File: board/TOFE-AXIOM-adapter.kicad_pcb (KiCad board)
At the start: 4 copper layers, 68.9 x 28.3 mm, 11 parts, among them CN1 C, U1 24AA01/24LC01B

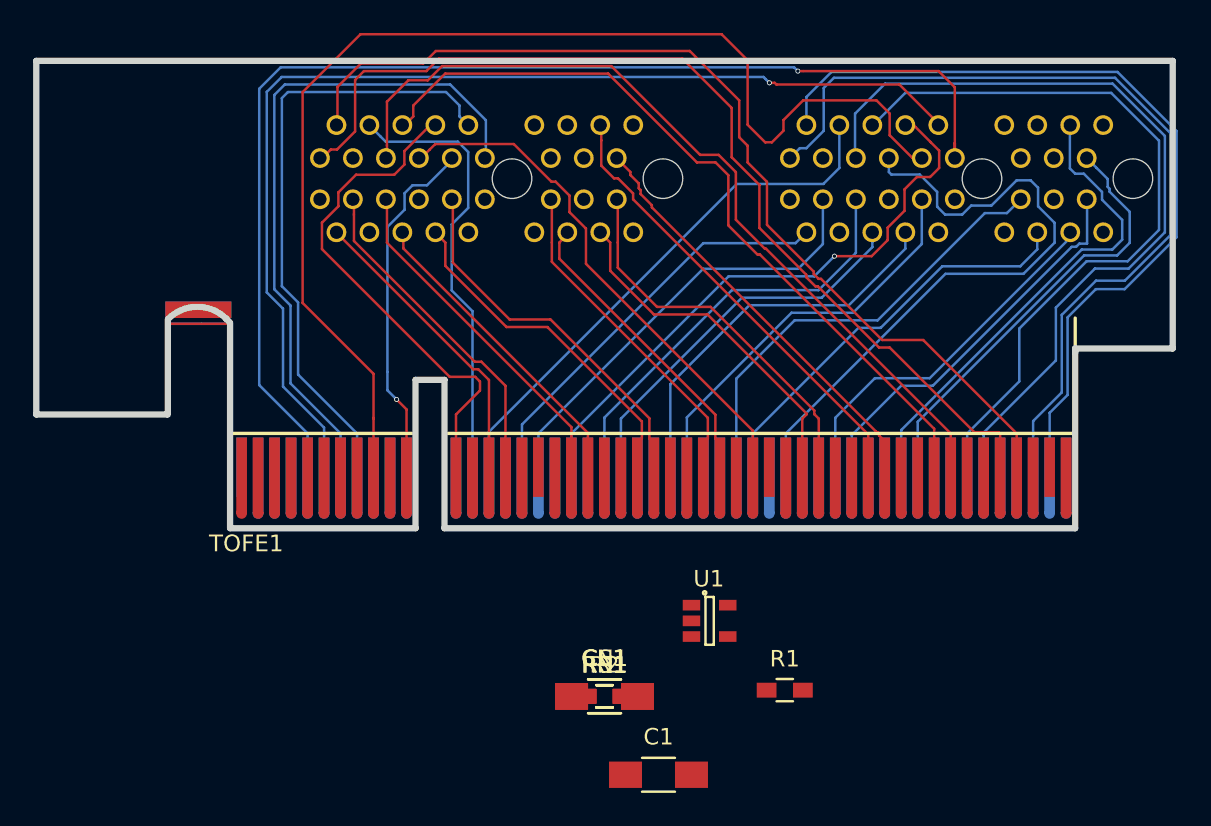
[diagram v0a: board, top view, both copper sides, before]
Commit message: More routing.
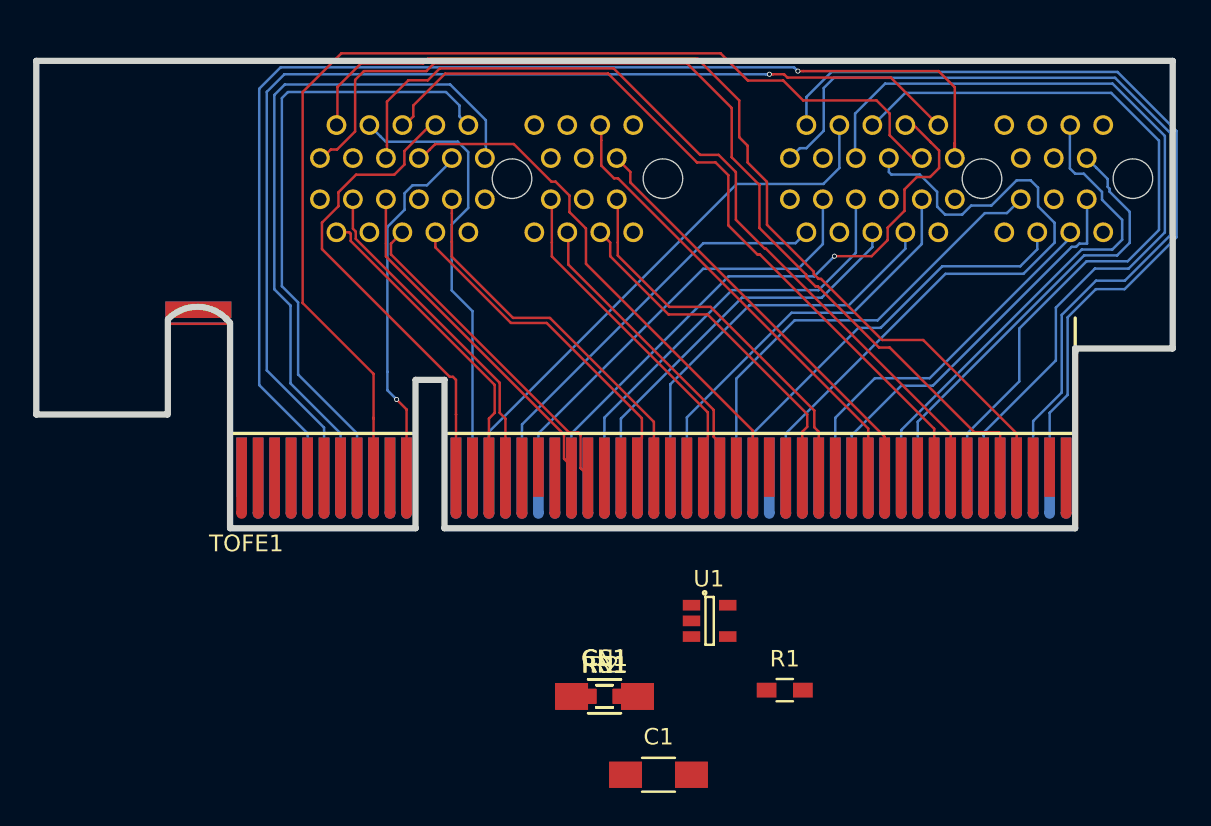
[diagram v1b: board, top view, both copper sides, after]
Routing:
- net /S_IO5: track 72.7 -> 67.0 mm
- net /VCC12V: track 2.30 -> 0.00 mm
- net /N_IO4: track 31.1 -> 29.2 mm
- net /N_LVDS_1_N: track 19.3 -> 20.3 mm
- net /N_LVDS_0_P: track 18.7 -> 19.3 mm
- net /N_SDA: track 61.2 -> 60.6 mm
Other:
- net class Default: clearance 0.2032 -> 0.1524
- rule trace_clearance: 0.2032 -> 0.1524
